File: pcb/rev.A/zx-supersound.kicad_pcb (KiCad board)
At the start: 2 copper layers, 170 x 63.6 mm, 163 parts, among them J1 PJ307, J2 PinHeader, J3 Conn_01x04, J4 Conn_02x31_Row_Letter_First, SW2 SW_DIP_x05, U1 MCP602, U10 YM3014B, U11 SAM2695, U12 AS6C4008-55SIN, U13 AMS1117-3.3, U14 SAA1099, U16 AMS1117-3.3, U17 NCP1117-5.0_TO252, U2 MCP602, U20 NCP1117-5.0_TO252, U21 NCP1117-5.0_TO252, U22 AS6C4008-55SIN, U23 74HC245, U3 Z84C0020PEC, U4 YM2203, U5 YM3014B, U6 MCP602, U7 EPM3256ATC144, U8 27C512, U9 YM2203, X1 32MHz

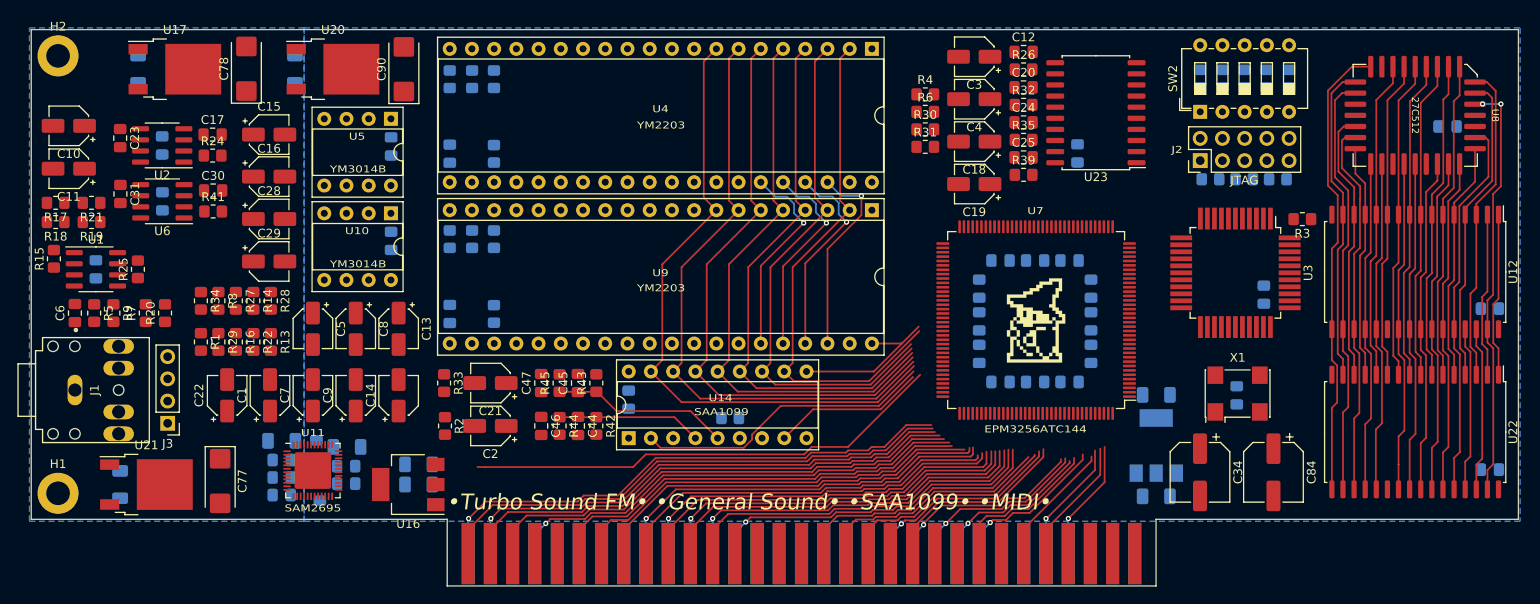
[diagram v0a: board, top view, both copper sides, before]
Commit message: wip pcb rev.A
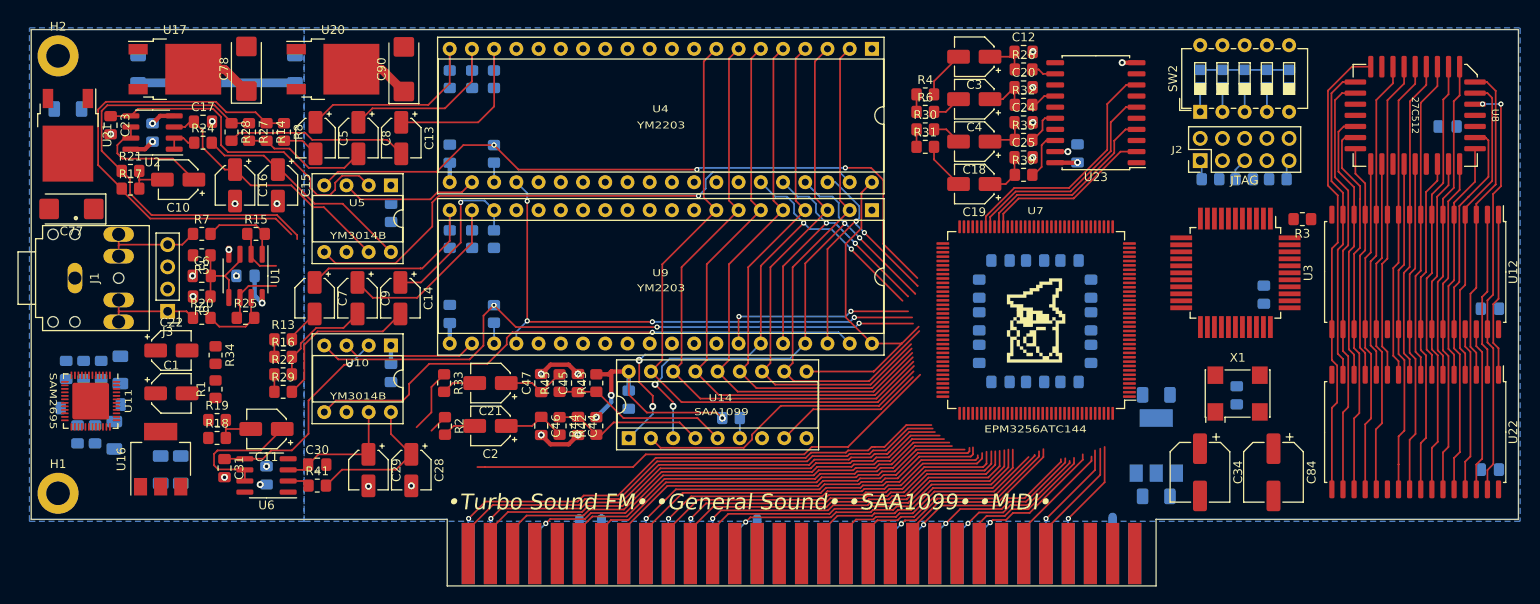
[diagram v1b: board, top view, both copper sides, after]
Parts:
- moved C92 43.3 mm to (62.8, 70.7), turned to 0 degrees
- moved U21 40.9 mm to (62.8, 73.7), turned to -90 degrees
- moved C11 37.4 mm to (85.5, 107.2)
- moved C77 35.4 mm to (63.2, 82.1), turned to 180 degrees
- moved C30 33.5 mm to (91.3, 111.3)
- moved C66 33.5 mm to (85.5, 112.6)
- moved U6 33.5 mm to (85.5, 112.6)
- moved C31 33.5 mm to (80.7, 111.7)
- moved R41 33.5 mm to (91.3, 113.7)
- moved C28 33.0 mm to (102.0, 112.0), turned to -90 degrees
- moved C69 31.2 mm to (63.9, 107.9), turned to 90 degrees
- moved R18 30.8 mm to (79.8, 108.3), turned to 0 degrees
- moved C68 30.1 mm to (63.0, 104.9), turned to 0 degrees
- moved C83 29.5 mm to (73.4, 111.9), turned to -90 degrees
- moved C32 28.9 mm to (65.9, 107.9), turned to 90 degrees
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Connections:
- R32 pad 2: Net-(R32-Pad2) -> Net-(U23-Pad14)
- R35 pad 2: Net-(R35-Pad2) -> Net-(U23-Pad16)
- R39 pad 2: Net-(R39-Pad2) -> Net-(U23-Pad18)
- R42 pad 2: +5VA -> +5VA_2
- R43 pad 2: +5VA -> +5VA_2
- R48 pad 2: +5VA -> +5VA_2
- U23 pad 11: Net-(R26-Pad2) -> unconnected-(U23-Pad11)
- U23 pad 12: unconnected-(U23-Pad12) -> Net-(R26-Pad2)
- U23 pad 13: Net-(R32-Pad2) -> unconnected-(U23-Pad13)
- U23 pad 14: unconnected-(U23-Pad14) -> Net-(U23-Pad14)
- U23 pad 15: Net-(R35-Pad2) -> unconnected-(U23-Pad15)
- U23 pad 16: unconnected-(U23-Pad16) -> Net-(U23-Pad16)
- U23 pad 17: Net-(R39-Pad2) -> unconnected-(U23-Pad17)
- U23 pad 18: unconnected-(U23-Pad18) -> Net-(U23-Pad18)
- U23 pad 2: unconnected-(U23-Pad2) -> /GDAC3
- U23 pad 3: /GDAC3 -> unconnected-(U23-Pad3)
- U23 pad 4: unconnected-(U23-Pad4) -> /GDAC2
- U23 pad 5: /GDAC2 -> unconnected-(U23-Pad5)
- U23 pad 6: unconnected-(U23-Pad6) -> /GDAC1
- U23 pad 7: /GDAC1 -> unconnected-(U23-Pad7)
- U23 pad 8: unconnected-(U23-Pad8) -> /GDAC0
- U23 pad 9: /GDAC0 -> unconnected-(U23-Pad9)
- U7 pad 80: /~{RST} -> /FM1_ENA
- U7 pad 81: /FM2_ENA -> /~{YM1_CS}
- U7 pad 82: /FM1_ENA -> /YM_M
- U7 pad 83: /~{YM1_CS} -> /AA0
- U7 pad 84: /~{YM2_CS} -> /~{ARD}
- U7 pad 87: /~{ARD} -> /~{YM2_CS}
- U7 pad 88: /AA0 -> /~{RST}
- U7 pad 90: /YM_M -> /FM2_ENA
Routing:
- net /FM1_ENA: track 0.00 -> 80.5 mm, vias 0 -> 3
- net /FM2_ENA: track 0.00 -> 73.8 mm, vias 0 -> 3
- net Net-(R19-Pad1): track 0.00 -> 69.0 mm
- net Net-(U4-Pad39): track 0.00 -> 67.6 mm, vias 0 -> 1
- net Net-(R1-Pad1): track 0.00 -> 66.8 mm
- net Net-(U10-Pad5): track 0.00 -> 65.5 mm, vias 0 -> 1
- net /~{RST}: track 0.00 -> 63.7 mm, vias 0 -> 4
- net /~{AWR}: track 23.3 -> 63.7 mm, vias 1 -> 4
- net Net-(C23-Pad1): track 0.00 -> 38.3 mm
- net /AA0: track 23.2 -> 61.3 mm, vias 1 -> 4
- net +5VA_2: track 0.00 -> 37.9 mm, vias 0 -> 3
- net GND: track 0.00 -> 33.1 mm, vias 0 -> 23
- net Net-(C16-Pad1): track 0.00 -> 29.8 mm
- net /GDAC0: track 0.00 -> 27.7 mm
- net Net-(C15-Pad1): track 0.00 -> 25.7 mm
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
